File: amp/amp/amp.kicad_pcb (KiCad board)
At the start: 2 copper layers, 50.8 x 53.3 mm, 7 parts, among them J1 Conn_01x02_Female, J2 TSJ3.5-009, J3 Screw_Terminal_01x02, J4 Screw_Terminal_01x02

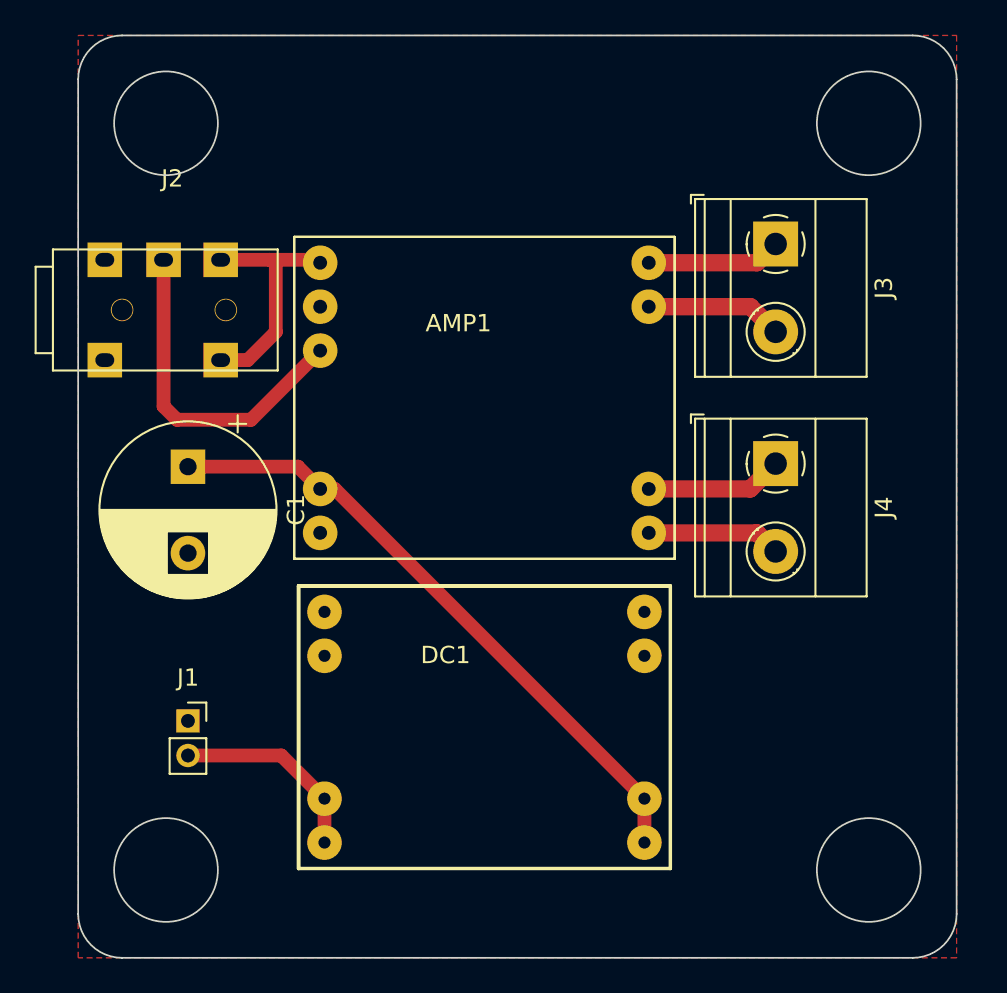
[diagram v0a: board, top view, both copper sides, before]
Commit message: Add projects
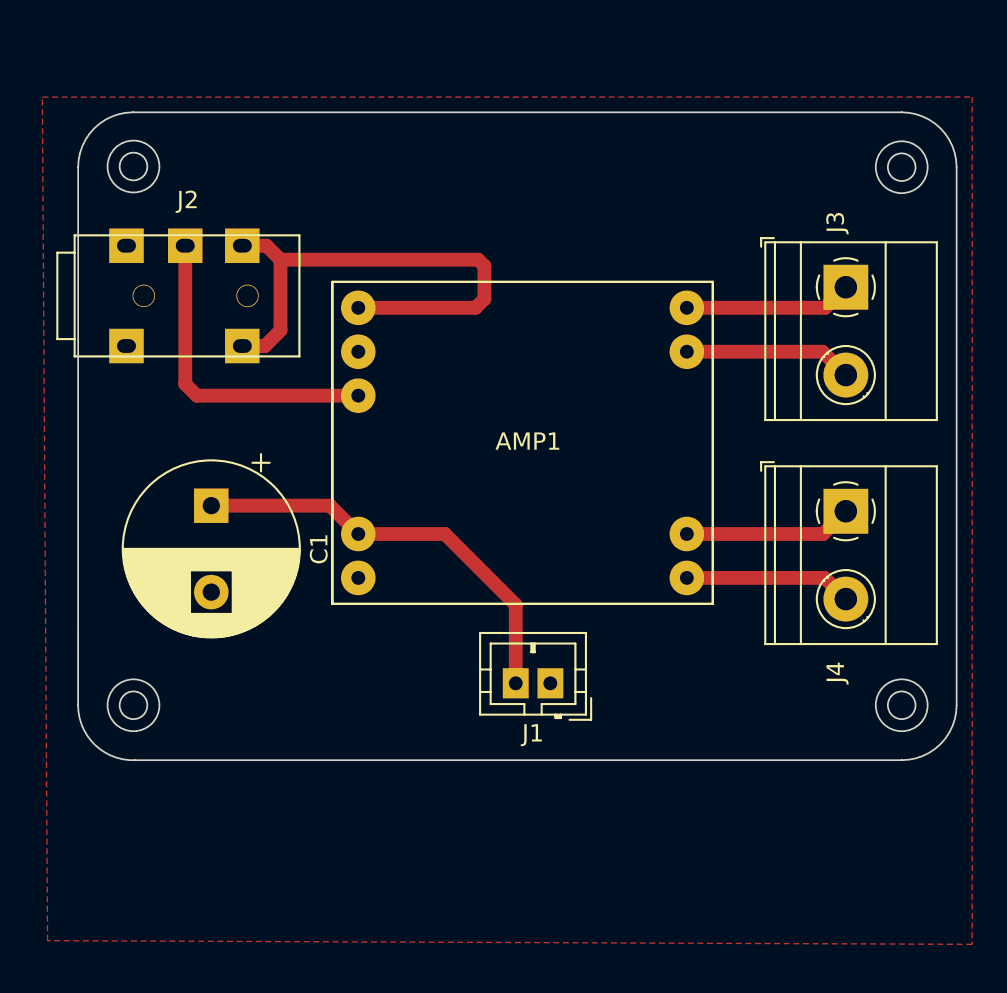
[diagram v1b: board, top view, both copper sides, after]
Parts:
- removed DC1: mp1584, _DC_DC:MP1584
- J1: value Conn_01x02_Female -> Conn_01x02; footprint Connector_PinSocket_2.00mm:PinSocket_1x02_P2.00mm_Vertical -> Connector_JST:JST_PH_B2B-PH-K_1x02_P2.00mm_Vertical
- moved J1 21.1 mm to (78.1, 65.4), turned to 180 degrees
- moved J4 4.91 mm to (95.2, 55.5)
- moved J3 4.77 mm to (95.2, 42.5)
- moved AMP1 3.41 mm to (67.0, 43.7)
- moved C1 2.63 mm to (58.5, 55.1)
- moved J2 1.50 mm to (49.6, 39.5)
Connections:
- J1 pad 2: Net-(DC1-Pad3) -> Net-(AMP1-Pad4)
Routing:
- net Net-(AMP1-Pad1): track 14.0 -> 31.1 mm
- net Net-(AMP1-Pad4): track 36.9 -> 24.5 mm
- net Net-(DC1-Pad3): track 11.5 -> 0.00 mm
- net Net-(AMP1-Pad9): track 7.79 -> 9.70 mm
- net Net-(AMP1-Pad6): track 7.79 -> 9.69 mm
- net Net-(AMP1-Pad7): track 7.94 -> 9.75 mm
- net Net-(AMP1-Pad8): track 7.95 -> 9.74 mm
- net Net-(AMP1-Pad3): track 19.5 -> 18.3 mm
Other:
- board size 50.8 x 53.3 mm -> 50.8 x 37.5 mm
